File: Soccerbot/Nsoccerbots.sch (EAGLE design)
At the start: 61 parts, among them IC1 33035P, X1 NXT-SOCKET, X2 NXT-SOCKET, X3 NXT-SOCKET, X4 NXT-SOCKET

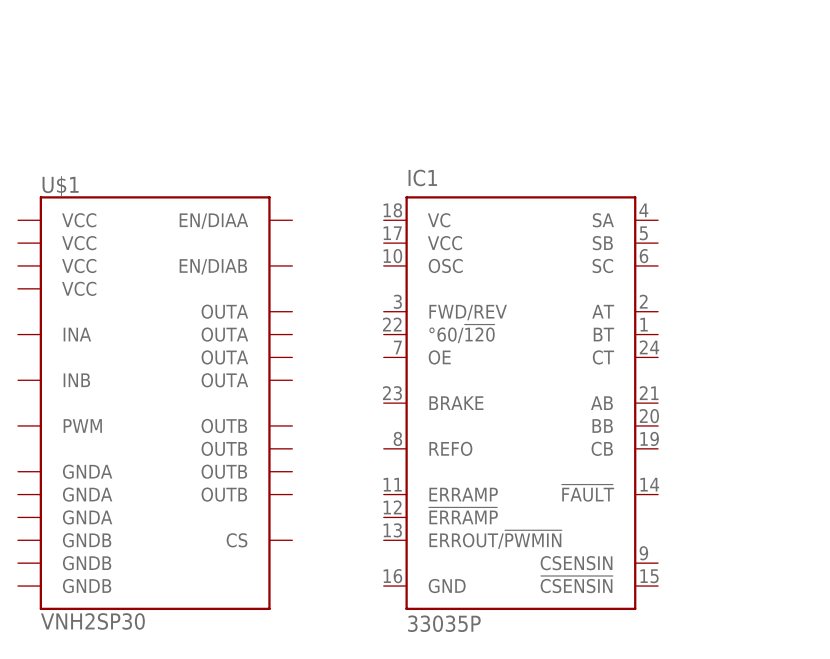
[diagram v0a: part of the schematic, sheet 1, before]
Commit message: M
Mm
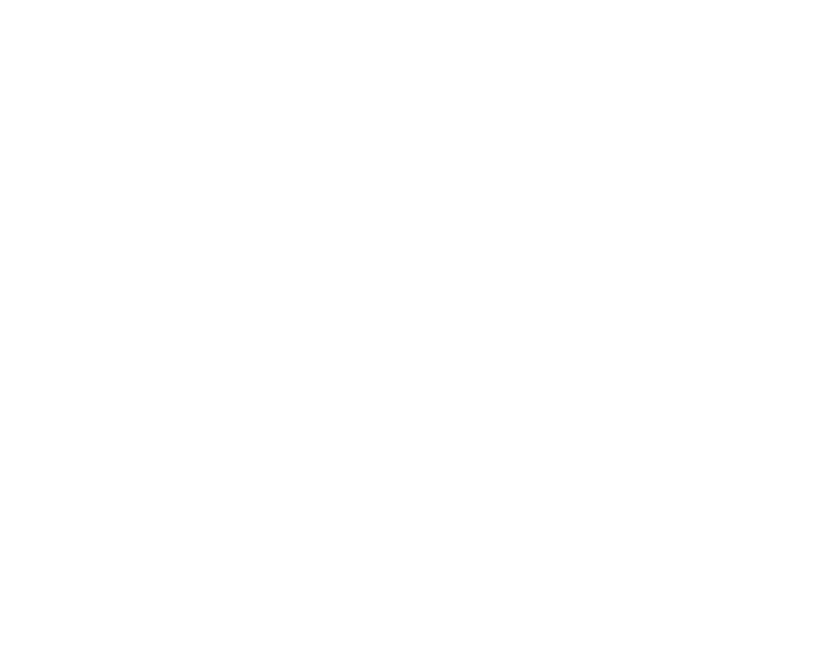
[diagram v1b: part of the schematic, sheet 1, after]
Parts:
- removed IC1: 33035P, motorola-sensor-driver:33035P
- removed U$1: VNH2SP30, SparkFun-IC-Special-Function:VNH2SP30
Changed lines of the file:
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@@
 <part name="ESC4P" library="con-wago-500" library_urn="urn:adsk.eagle:library:195" deviceset="W237-102" device=""/>
 <part name="BATERY" library="con-wago-500" library_urn="urn:adsk.eagle:library:195" deviceset="W237-102" device=""/>
-<part name="U$1" library="SparkFun-IC-Special-Function" deviceset="VNH2SP30" device=""/>
-<part name="IC1" library="motorola-sensor-driver" deviceset="*33035" device="P"/>
 </parts>
 <sheets>
@@
 <instance part="BATERY" gate="-1" x="-228.6" y="66.04"/>
 <instance part="BATERY" gate="-2" x="-228.6" y="60.96"/>
-<instance part="U$1" gate="G$1" x="-256.54" y="5.08"/>
-<instance part="IC1" gate="G$1" x="-215.9" y="5.08"/>
 </instances>
 <busses>

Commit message: s
S
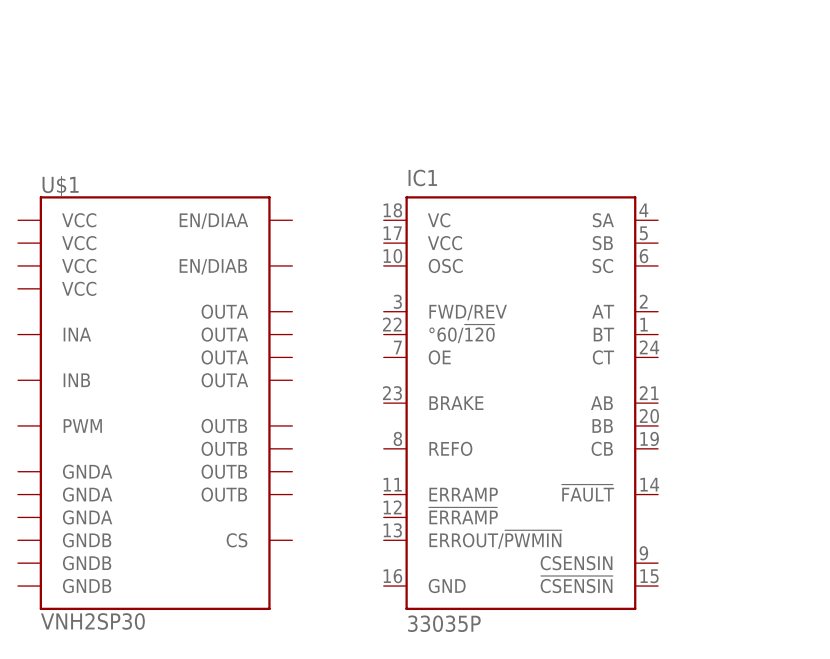
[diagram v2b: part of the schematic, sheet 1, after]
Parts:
- added IC1: 33035P, motorola-sensor-driver:33035P
- added U$1: VNH2SP30, SparkFun-IC-Special-Function:VNH2SP30
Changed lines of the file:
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@@
 <part name="ESC4P" library="con-wago-500" library_urn="urn:adsk.eagle:library:195" deviceset="W237-102" device=""/>
 <part name="BATERY" library="con-wago-500" library_urn="urn:adsk.eagle:library:195" deviceset="W237-102" device=""/>
+<part name="U$1" library="SparkFun-IC-Special-Function" deviceset="VNH2SP30" device=""/>
+<part name="IC1" library="motorola-sensor-driver" deviceset="*33035" device="P"/>
 </parts>
 <sheets>
@@
 <instance part="BATERY" gate="-1" x="-228.6" y="66.04"/>
 <instance part="BATERY" gate="-2" x="-228.6" y="60.96"/>
+<instance part="U$1" gate="G$1" x="-256.54" y="5.08"/>
+<instance part="IC1" gate="G$1" x="-215.9" y="5.08"/>
 </instances>
 <busses>
